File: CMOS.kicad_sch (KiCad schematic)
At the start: 11 parts, among them U21 28F010, U210 74LS138, U211 74AUC2G04, U22 28F010, U23 28F010, U24 28F010, U25 28F010, U26 28F010, U27 28F010, U28 28F010, U29 74LS138

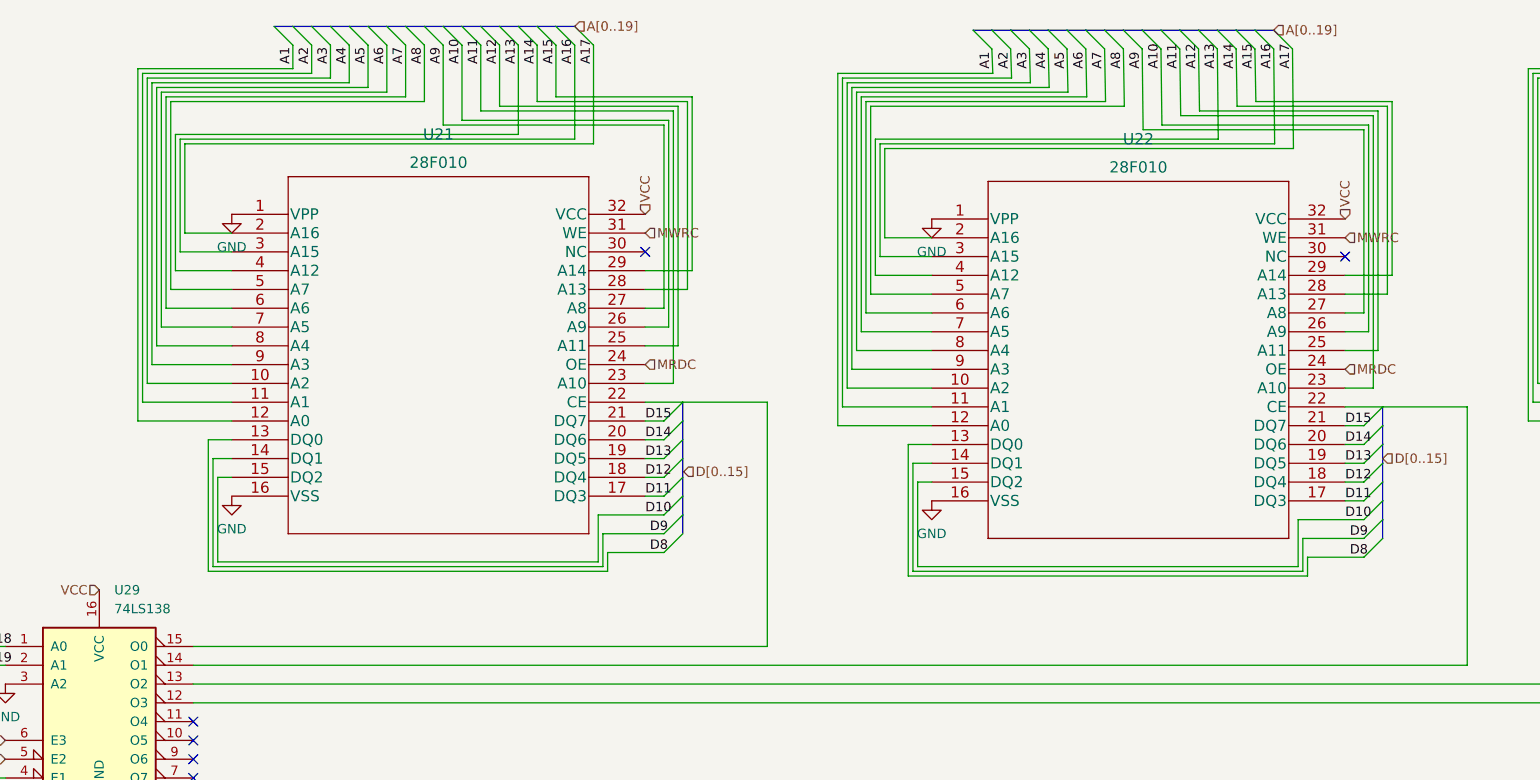
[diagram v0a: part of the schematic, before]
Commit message: Added bullet 6
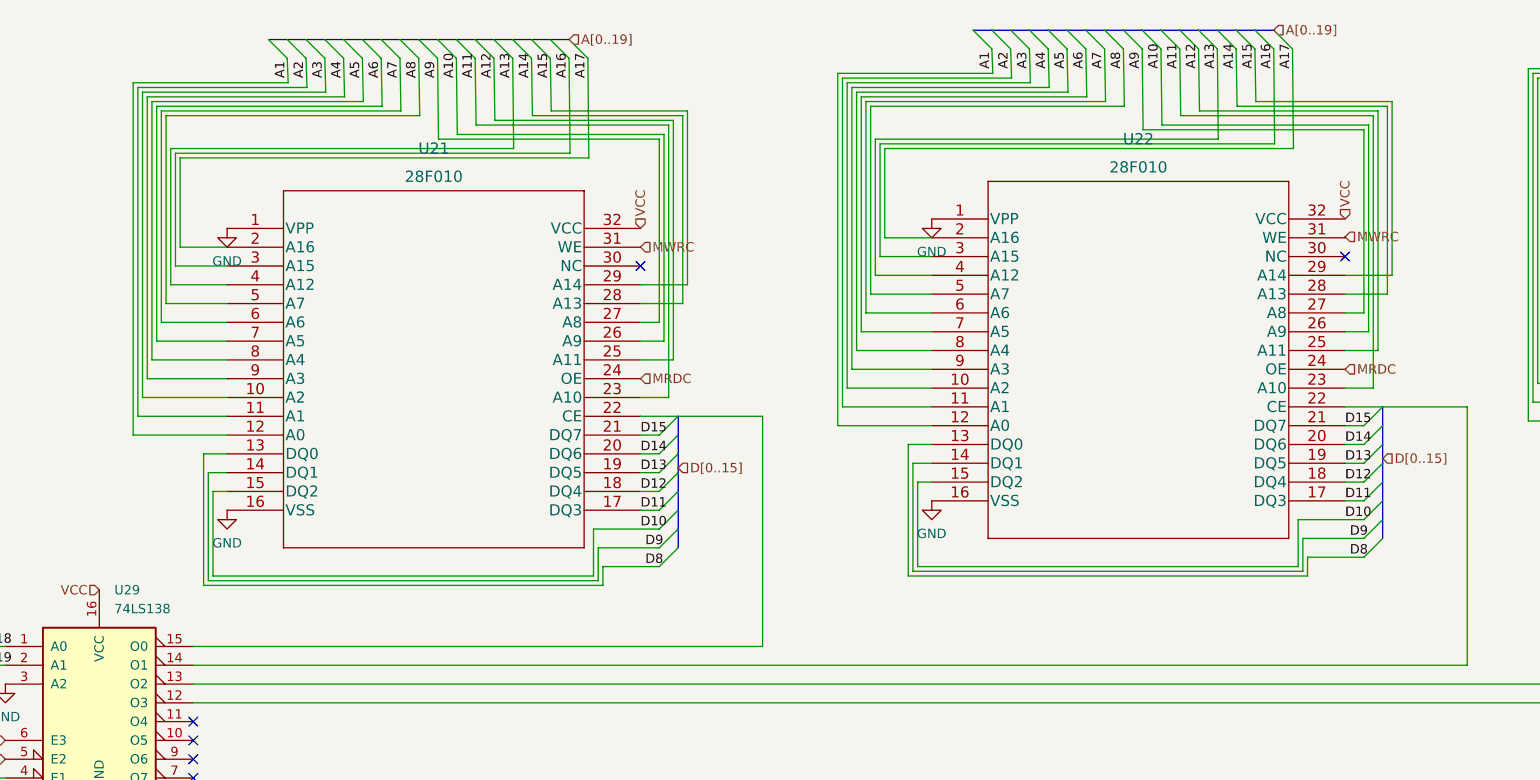
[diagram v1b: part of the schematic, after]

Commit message: stuff
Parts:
- removed U210, U29: 74LS138, symbol 74xx:74LS138
- removed U211: 74AUC2G04, symbol 74xGxx:74AUC2G04
- removed U23, U24, U25, U26, U27, U28: 28F010, parts:28F010, symbol 28F010:28F010
- added U23: 74LS138, symbol 74xx:74LS138
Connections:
- net A0: now also U23.3 (A2)
- net A18: now also U23.1 (A0)
- net A19: now also U23.2 (A1)
- net BHE: now also U23.5 (E2)
- net GND: now also U23.4 (E1), U23.8 (GND)
- net M/IO: now also U23.6 (E3)
- net VCC: now also U23.16 (VCC)
- net at U22.22 (CE): now also U21.22 (CE), U23.7 (O7)
- net MRDC renamed MRD
- net MWRC renamed MWR
- no-connect marks 16 -> 9
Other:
- moved on the sheet: U21
